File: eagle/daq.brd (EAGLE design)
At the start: 59.7 x 65.4 mm, 77 parts

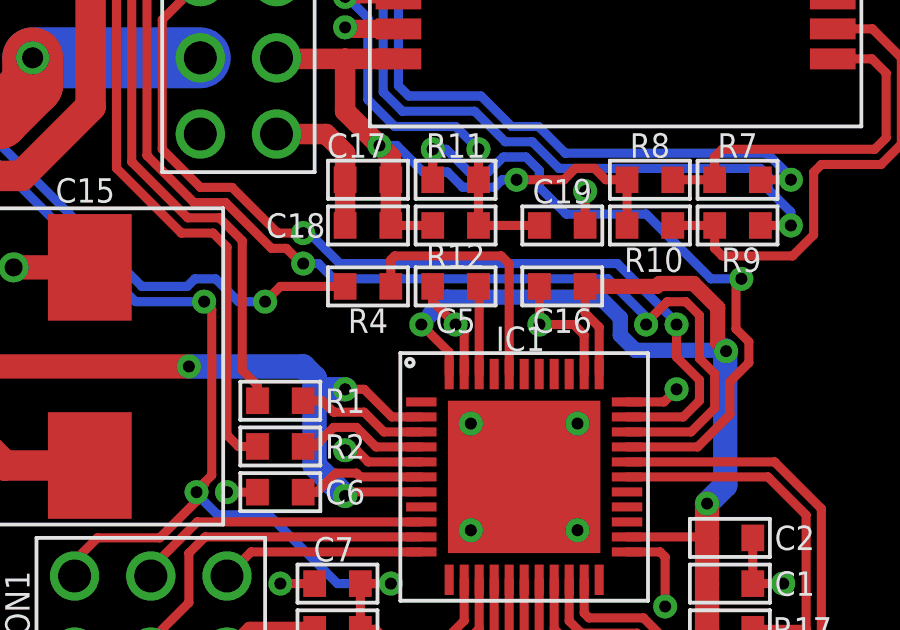
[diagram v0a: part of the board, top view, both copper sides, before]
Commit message: do
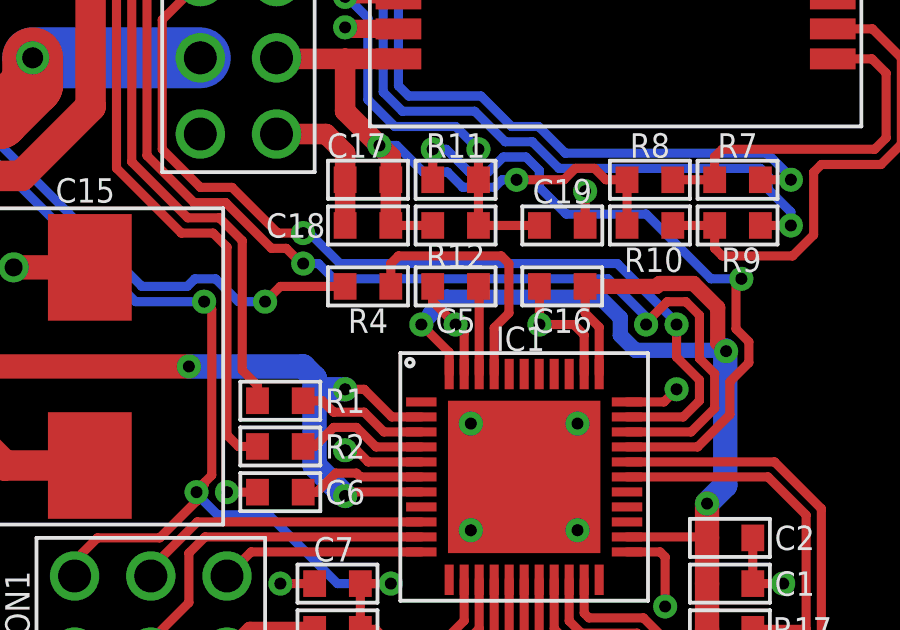
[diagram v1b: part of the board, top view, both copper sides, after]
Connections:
- net N$1: now also IC1.41; no longer IC1.40
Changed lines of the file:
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@@
 </polygon>
-</signal>
-<signal name="N$1">
-<contactref element="IC1" pad="40"/>
-<contactref element="R4" pad="1"/>
-<wire x1="33.79" y1="42.791" x2="33.528" y2="43.053" width="0.3048" layer="1"/>
-<wire x1="33.528" y1="43.053" x2="29.972" y2="43.053" width="0.3048" layer="1"/>
-<wire x1="29.845" y1="42.926" x2="29.845" y2="42.037" width="0.3048" layer="1"/>
-<wire x1="33.79" y1="39.116" x2="33.79" y2="42.791" width="0.3048" layer="1"/>
-<wire x1="29.972" y1="43.053" x2="29.845" y2="42.926" width="0.3048" layer="1"/>
 </signal>
 <signal name="N$17" airwireshidden="yes">
@@
 <wire x1="46.101" y1="26.43405625" x2="44.45" y2="28.08505625" width="0.3048" layer="1"/>
 </signal>
+<signal name="N$1">
+<contactref element="R4" pad="1"/>
+<contactref element="IC1" pad="41"/>
+<wire x1="29.845" y1="42.037" x2="29.845" y2="42.799" width="0.3048" layer="1"/>
+<wire x1="29.845" y1="42.799" x2="30.099" y2="43.053" width="0.3048" layer="1"/>
+<wire x1="30.099" y1="43.053" x2="33.528" y2="43.053" width="0.3048" layer="1"/>
+<wire x1="33.528" y1="43.053" x2="33.782" y2="42.799" width="0.3048" layer="1"/>
+<wire x1="33.782" y1="41.148" x2="33.782" y2="42.799" width="0.3048" layer="1"/>
+<wire x1="33.29" y1="39.116" x2="33.29" y2="40.656" width="0.3048" layer="1"/>
+<wire x1="33.29" y1="40.656" x2="33.782" y2="41.148" width="0.3048" layer="1"/>
+</signal>
 </signals>
